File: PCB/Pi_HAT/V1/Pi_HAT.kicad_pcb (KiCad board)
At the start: 2 copper layers, 59 x 69.6 mm, 19 parts, among them J1 MPU9250, J2 Pi_GPIO, J3 Display, J4 Solenoid I2C, J5 XT60PW-M, J6 Solenoid I2C

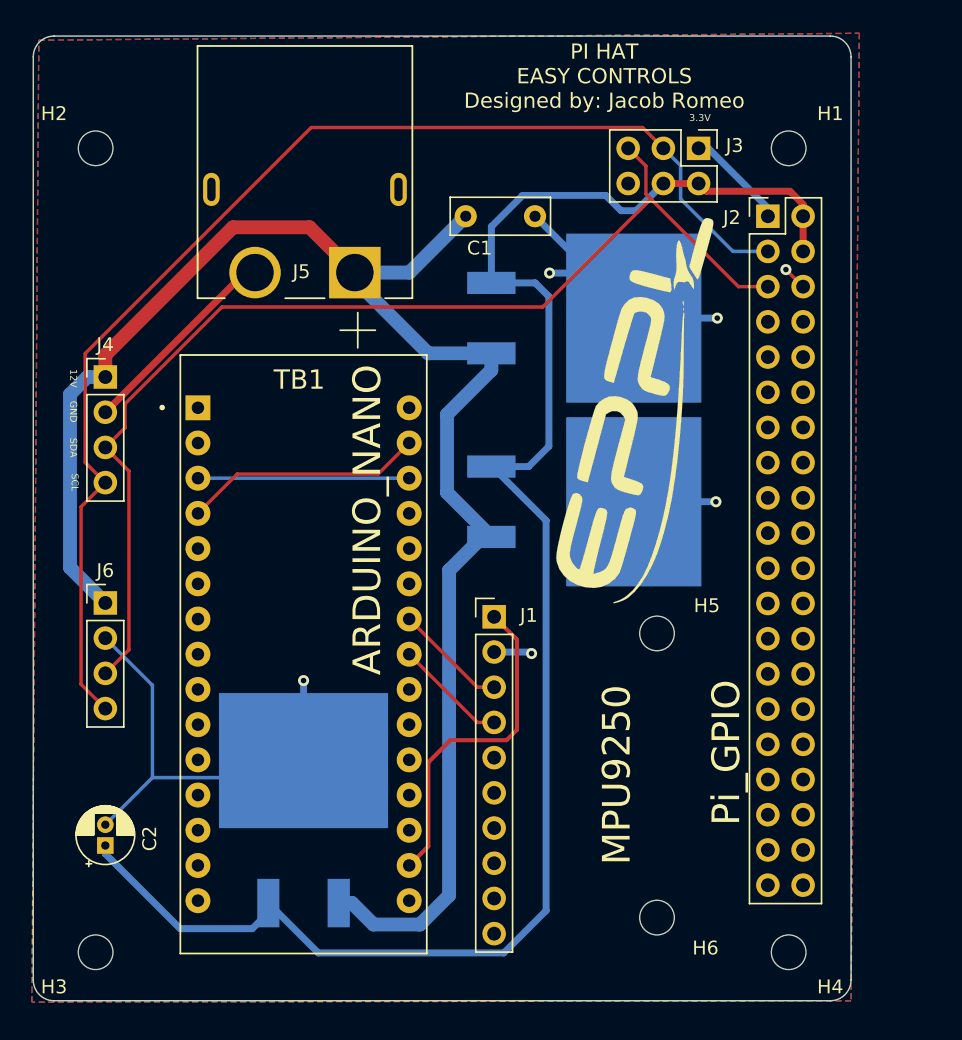
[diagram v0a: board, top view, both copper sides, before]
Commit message: Updated V1 Pi Hat
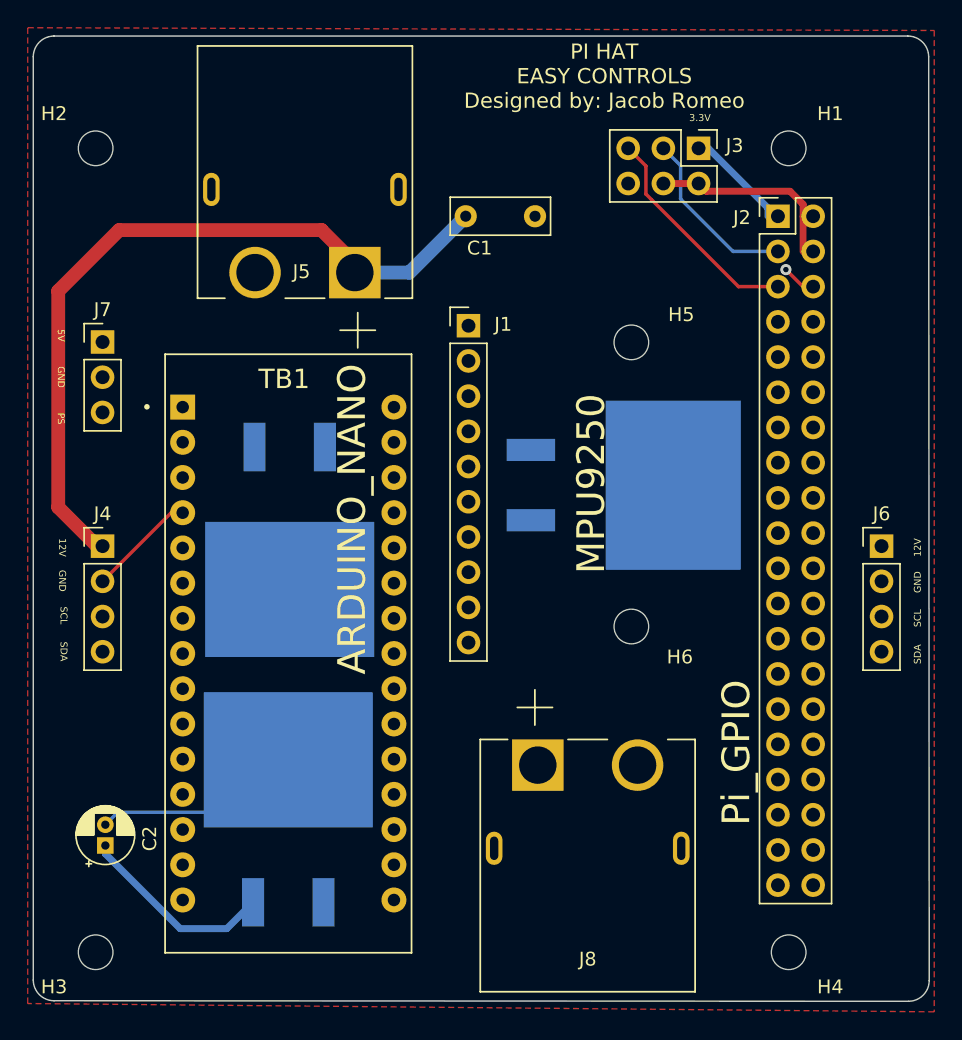
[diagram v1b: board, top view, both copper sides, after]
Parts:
- removed G***: LOGO, .pretty:eppl_logo
- added J7: Pressure, Connector_PinHeader_2.54mm:PinHeader_1x03_P2.54mm_Vertical, F.Cu at (103.0, 88.5)
- added J8: XT60PW-M, .pretty:AMASS_XT60PW-M, F.Cu at (138.0, 125.0)
- moved J6 56.1 mm to (159.2, 103.2)
- moved VR2 21.4 mm to (116.5, 102.8), turned to -90 degrees
- moved H5 21.1 mm to (141.2, 88.5)
- moved H6 21.1 mm to (141.2, 109.0)
- moved J1 21.1 mm to (129.4, 87.3)
- moved VR1 12.4 mm to (140.6, 98.8)
- moved J4 12.2 mm to (103.0, 103.2)
- moved TB1 1.10 mm to (116.4, 111.0)
- moved VR3 1.10 mm to (116.4, 122.2)
- moved J2 0.72 mm to (151.7, 79.4)
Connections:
- TB1 pad 19: unconnected-(TB1-Pad19) -> /PS
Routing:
- net /5V: track 125.2 -> 28.4 mm
- net /SDA: track 88.8 -> 12.0 mm
- net GND: track 99.9 -> 24.7 mm, vias 6 -> 1
- net /SCL: track 80.9 -> 15.4 mm
- net 12V: track 119.1 -> 54.5 mm
- net 3.3VN: track 24.2 -> 0.00 mm
- net unconnected-(TB1-Pad28): track 15.2 -> 0.00 mm
- net SDAN: track 8.17 -> 0.00 mm
- net SCLN: track 8.17 -> 0.00 mm
- removed copper zone on B.Cu, net GND
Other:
- board size 59 x 69.6 mm -> 64.6 x 69.6 mm
- board text added: "5V"
- board text added: "PS"
